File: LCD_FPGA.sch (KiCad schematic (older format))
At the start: 8 parts

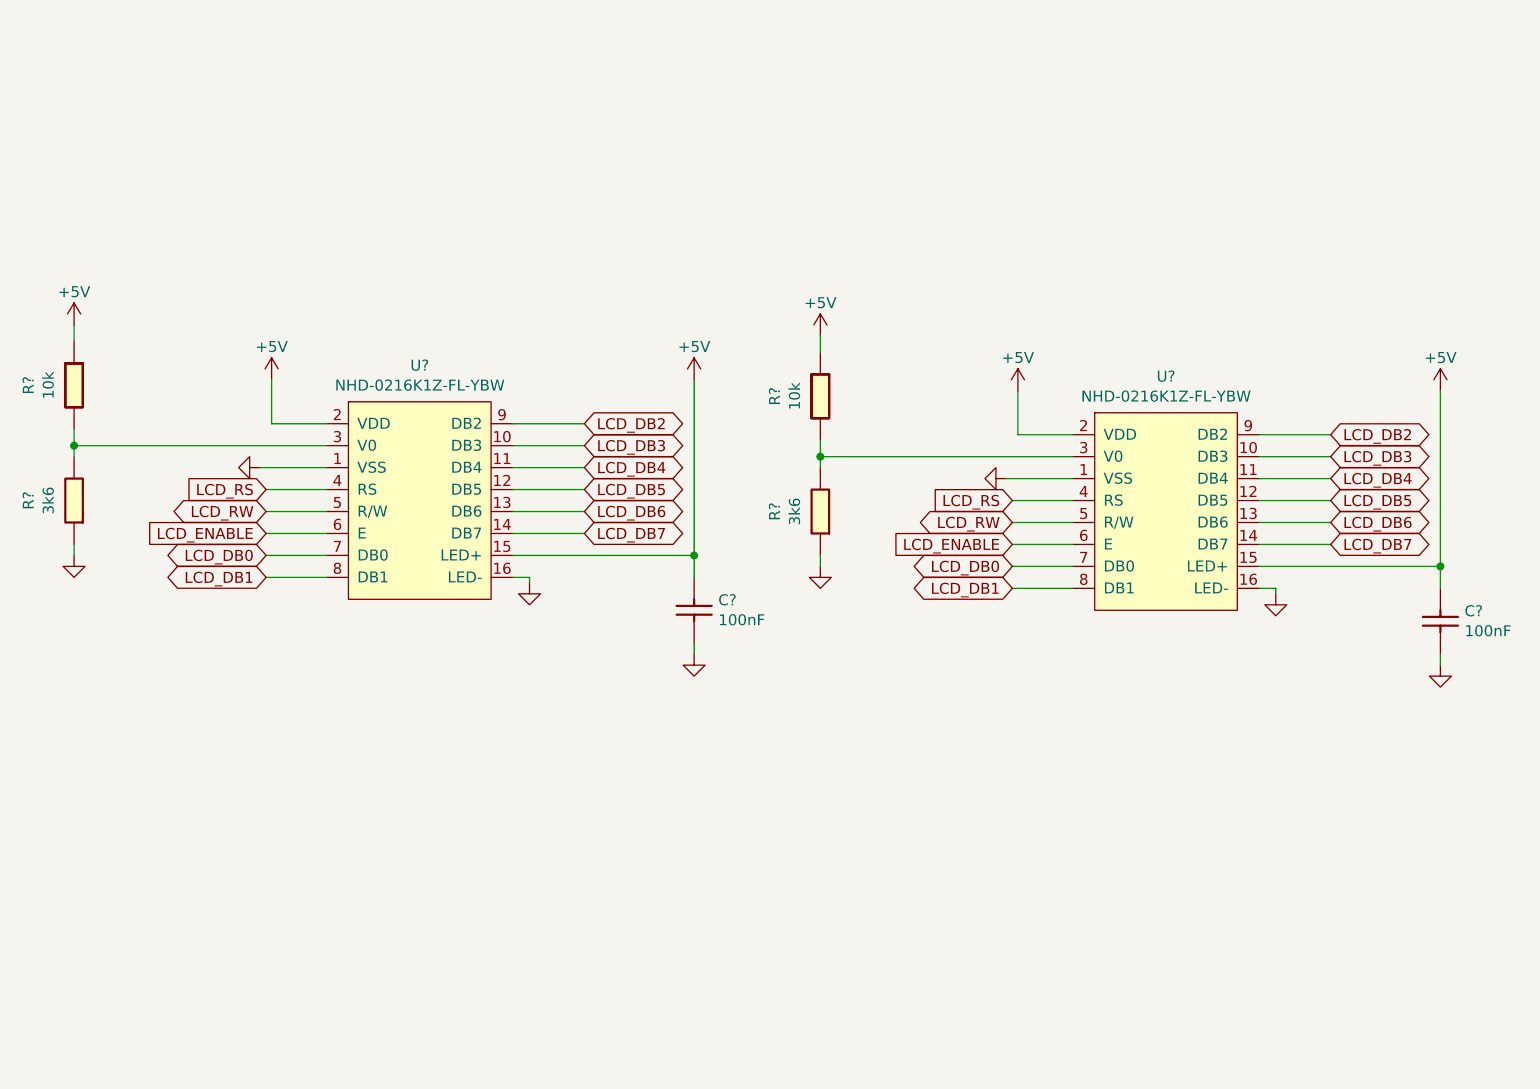
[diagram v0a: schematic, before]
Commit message: More fixing up of the FPGA symbols, lashed up the sigma delta A/D converter circuitry.  Fixed up the LCD page.  Two displays, two separate enables needed here folks.  FPGA I/O banks power supplies' needs another looking at.  Still lots of stuff to clean up here...
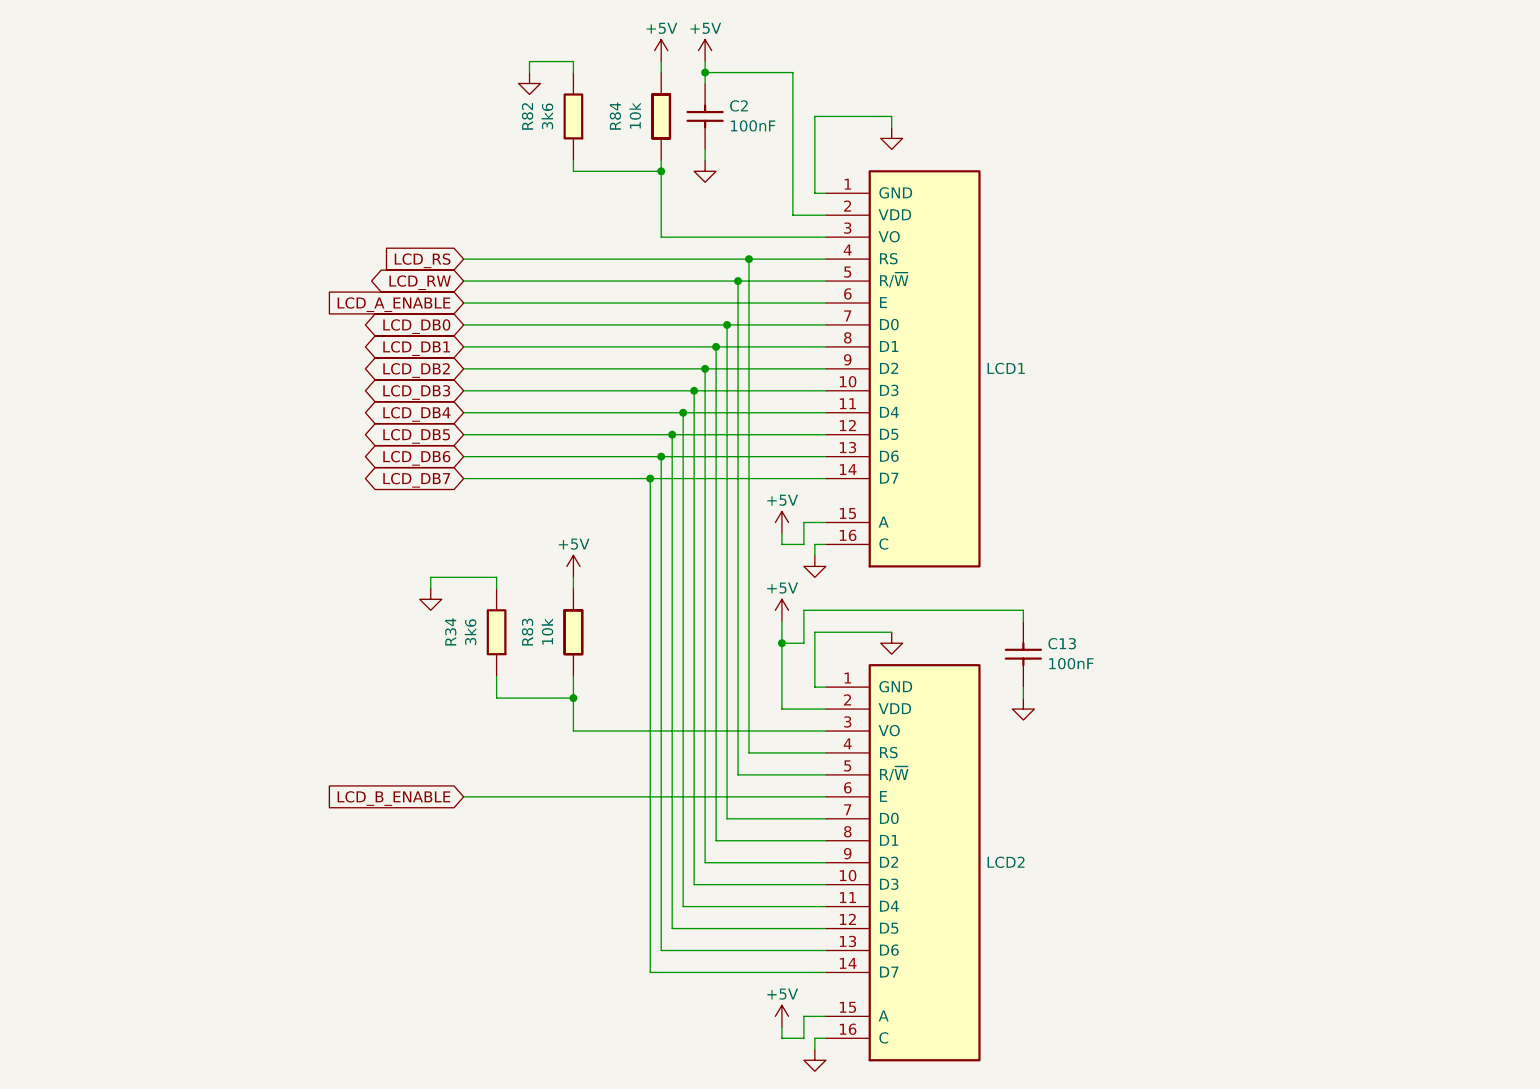
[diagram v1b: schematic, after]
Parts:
- removed U? (x2): NHD-0216K1Z-FL-YBW, symbol OpenVent:NHD-0216K1Z-FL-YBW
- added LCD1, LCD2: LCD_MOD_32DIG_16X2_TRANS_YLW_GRN, symbol OpenVent:LCD_MOD_32DIG_16X2_TRANS_YLW_GRN
- gave numbers to parts that had none: 6
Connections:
- net +5V: now also LCD1.15 (A), LCD1.2 (VDD), LCD2.15 (A), LCD2.2 (VDD)
- net GND: now also R34.2, R82.2, LCD1.1 (GND), LCD1.16 (C), LCD2.1 (GND), LCD2.16 (C); no longer R34.1, R82.1
- net LCD_DB0: now also LCD1.7 (D0), LCD2.7 (D0)
- net LCD_DB1: now also LCD1.8 (D1), LCD2.8 (D1)
- net LCD_DB2: now also LCD1.9 (D2), LCD2.9 (D2)
- net LCD_DB3: now also LCD1.10 (D3), LCD2.10 (D3)
- net LCD_DB4: now also LCD1.11 (D4), LCD2.11 (D4)
- net LCD_DB5: now also LCD1.12 (D5), LCD2.12 (D5)
- net LCD_DB6: now also LCD1.13 (D6), LCD2.13 (D6)
- net LCD_DB7: now also LCD1.14 (D7), LCD2.14 (D7)
- net LCD_RS: now also LCD1.4 (RS), LCD2.4 (RS)
- net LCD_RW: now also LCD1.5 (R/~W), LCD2.5 (R/~W)
- net at R84.1: now also R82.1, LCD1.3 (VO); no longer R82.2
- net at R83.1: now also R34.1, LCD2.3 (VO); no longer R34.2
- new net LCD_A_ENABLE: LCD1.6 (E)
- new net LCD_B_ENABLE: LCD2.6 (E)
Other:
- moved on the sheet: C13, C2, R34, R82, R83, R84
